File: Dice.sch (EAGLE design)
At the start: 14 parts, among them IC1 PIC12F629SN

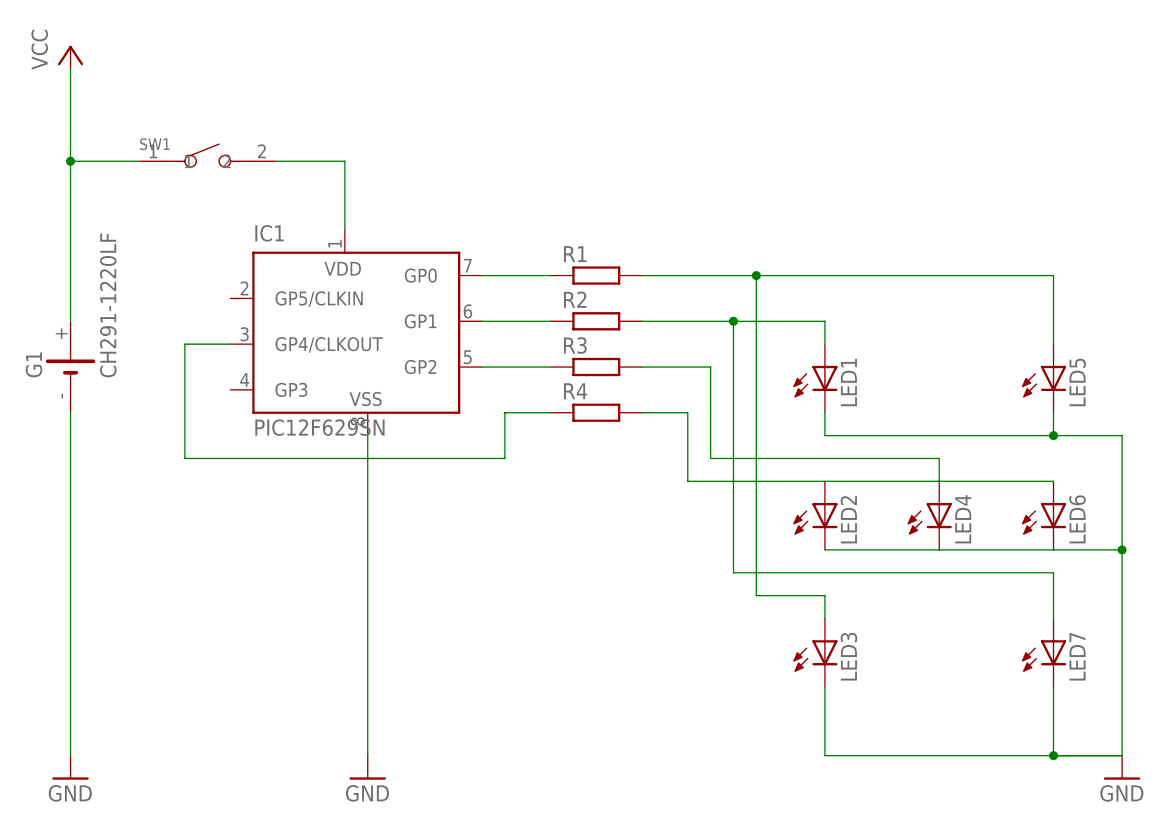
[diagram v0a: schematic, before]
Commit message: Always powered
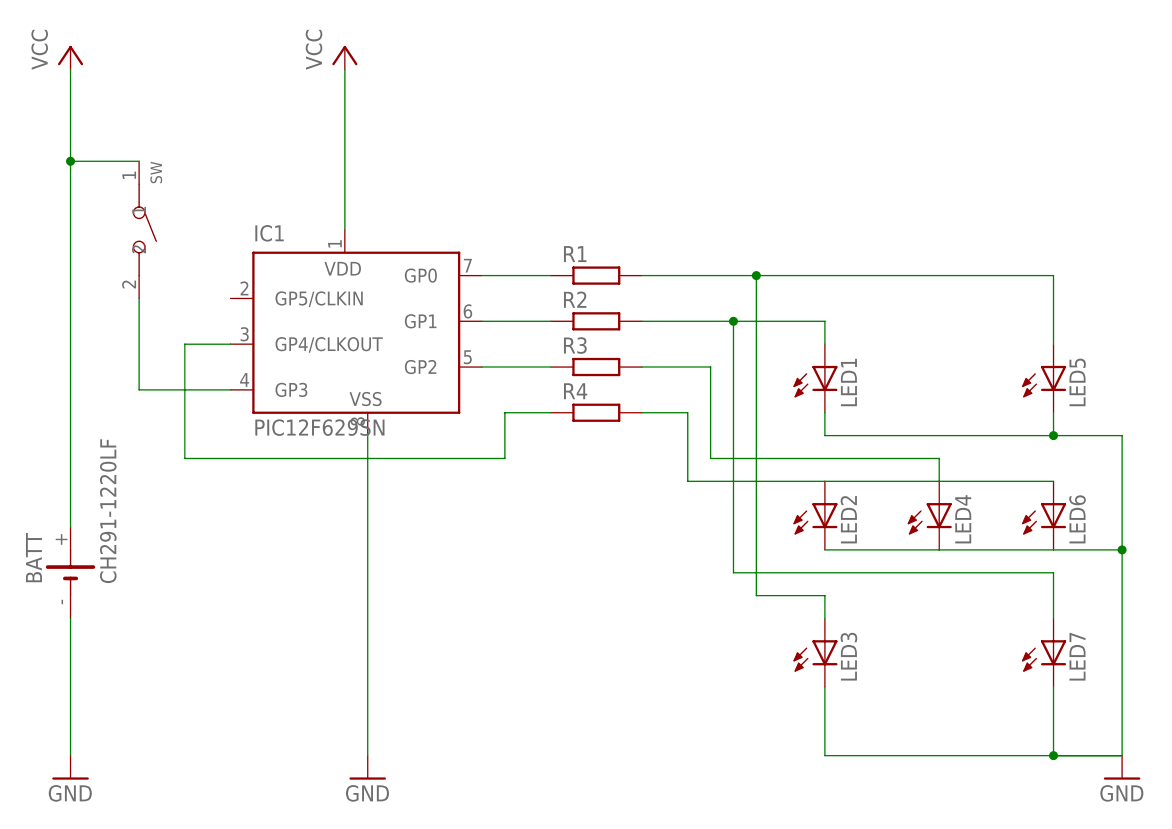
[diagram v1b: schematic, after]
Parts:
- removed G1: CH291-1220LF, battery:CH291-1220LF
- removed SW1: (no value), Seeed-OPL-Switch:SMD-BUTTON(2P-6.0X3.0X2.5MM)-DHT-1163S
- added BATT: CH291-1220LF, battery:CH291-1220LF
- added SW: (no value), Seeed-OPL-Switch:SMD-BUTTON(2P-6.0X3.0X2.5MM)-DHT-1163S
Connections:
- net N$11 renamed LED4
- net N$12 renamed LED2&6
- net N$2 renamed GP0
- net N$3 renamed GP1
- net N$4 renamed GP2
- net N$5 renamed GP4
- net N$6 renamed LED3&5
- net N$7 renamed LED1&7
- removed net N$1: IC1.VDD, SW1.2
- new net GP3: IC1.GP3, SW.2
- net GND: now also BATT.-; no longer G1.-
- net VCC: now also BATT.+, IC1.VDD, SW.1; no longer G1.+, SW1.1
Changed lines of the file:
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@@
 </classes>
 <parts>
-<part name="G1" library="battery" deviceset="CH291-1220LF" device=""/>
+<part name="BATT" library="battery" deviceset="CH291-1220LF" device=""/>
 <part name="GND1" library="supply1" deviceset="GND" device=""/>
 <part name="P+1" library="supply1" deviceset="VCC" device=""/>
@@
 <part name="R3" library="resistor" deviceset="R-EU_" device="R0805"/>
 <part name="R4" library="resistor" deviceset="R-EU_" device="R0805"/>
-<part name="SW1" library="Seeed-OPL-Switch" deviceset="SMD-BUTTON(2P-6.0X3.0X2.5MM)" device="-DHT-1163S"/>
+<part name="SW" library="Seeed-OPL-Switch" deviceset="SMD-BUTTON(2P-6.0X3.0X2.5MM)" device="-DHT-1163S"/>
 <part name="GND2" library="supply1" deviceset="GND" device=""/>
 <part name="GND3" library="supply1" deviceset="GND" device=""/>
+<part name="P+2" library="supply1" deviceset="VCC" device=""/>
 </parts>
 <sheets>
@@
 </plain>
 <instances>
-<instance part="G1" gate="G1" x="22.86" y="58.42" rot="R90"/>
+<instance part="BATT" gate="G1" x="22.86" y="35.56" rot="R90"/>
 <instance part="GND1" gate="1" x="22.86" y="12.7"/>
 <instance part="P+1" gate="VCC" x="22.86" y="93.98"/>
@@
 <instance part="R3" gate="G$1" x="81.28" y="58.42"/>
 <instance part="R4" gate="G$1" x="81.28" y="53.34"/>
-<instance part="SW1" gate="G$1" x="38.1" y="81.28"/>
+<instance part="SW" gate="G$1" x="30.48" y="73.66" rot="R270"/>
 <instance part="GND2" gate="1" x="55.88" y="12.7"/>
 <instance part="GND3" gate="1" x="139.7" y="12.7"/>
+<instance part="P+2" gate="VCC" x="53.34" y="93.98"/>
 </instances>
 <busses>
@@
 <segment>
 <pinref part="P+1" gate="VCC" pin="VCC"/>
-<pinref part="G1" gate="G1" pin="+"/>
+<pinref part="BATT" gate="G1" pin="+"/>
 <wire x1="22.86" y1="91.44" x2="22.86" y2="81.28" width="0.1524" layer="91"/>
-<pinref part="SW1" gate="G$1" pin="1"/>
-<wire x1="22.86" y1="81.28" x2="22.86" y2="63.5" width="0.1524" layer="91"/>
+<pinref part="SW" gate="G$1" pin="1"/>
+<wire x1="22.86" y1="81.28" x2="22.86" y2="40.64" width="0.1524" layer="91"/>
 <wire x1="22.86" y1="81.28" x2="30.48" y2="81.28" width="0.1524" layer="91"/>
 <junction x="22.86" y="81.28"/>
+</segment>
+<segment>
+<pinref part="P+2" gate="VCC" pin="VCC"/>
+<pinref part="IC1" gate="G$1" pin="VDD"/>
+<wire x1="53.34" y1="91.44" x2="53.34" y2="73.66" width="0.1524" layer="91"/>
 </segment>
 </net>
 <net name="GND" class="0">
 <segment>
-<pinref part="G1" gate="G1" pin="-"/>
+<pinref part="BATT" gate="G1" pin="-"/>
 <pinref part="GND1" gate="1" pin="GND"/>
-<wire x1="22.86" y1="53.34" x2="22.86" y2="15.24" width="0.1524" layer="91"/>
+<wire x1="22.86" y1="30.48" x2="22.86" y2="15.24" width="0.1524" layer="91"/>
 </segment>
 <segment>
@@
 </segment>
 </net>
-<net name="N$1" class="0">
+<net name="GP3" class="0">
 <segment>
-<pinref part="SW1" gate="G$1" pin="2"/>
-<pinref part="IC1" gate="G$1" pin="VDD"/>
-<wire x1="45.72" y1="81.28" x2="53.34" y2="81.28" width="0.1524" layer="91"/>
-<wire x1="53.34" y1="81.28" x2="53.34" y2="73.66" width="0.1524" layer="91"/>
+<pinref part="SW" gate="G$1" pin="2"/>
+<wire x1="30.48" y1="66.04" x2="30.48" y2="55.88" width="0.1524" layer="91"/>
+<pinref part="IC1" gate="G$1" pin="GP3"/>
+<wire x1="30.48" y1="55.88" x2="40.64" y2="55.88" width="0.1524" layer="91"/>
 </segment>
 </net>
-<net name="N$2" class="0">
+<net name="GP0" class="0">
 <segment>
 <pinref part="IC1" gate="G$1" pin="GP0"/>
@@
 </segment>
 </net>
-<net name="N$3" class="0">
+<net name="GP1" class="0">
 <segment>
 <pinref part="IC1" gate="G$1" pin="GP1"/>
@@
 </segment>
 </net>
-<net name="N$4" class="0">
+<net name="GP2" class="0">
 <segment>
 <pinref part="IC1" gate="G$1" pin="GP2"/>
@@
 </segment>
 </net>
-<net name="N$5" class="0">
+<net name="GP4" class="0">
 <segment>
 <pinref part="IC1" gate="G$1" pin="GP4/CLKOUT"/>
@@
 </segment>
 </net>
-<net name="N$6" class="0">
+<net name="LED3&amp;5" class="0">
 <segment>
 <pinref part="R1" gate="G$1" pin="2"/>
@@
 </segment>
 </net>
-<net name="N$7" class="0">
+<net name="LED1&amp;7" class="0">
 <segment>
 <pinref part="R2" gate="G$1" pin="2"/>
@@
 </segment>
 </net>
-<net name="N$11" class="0">
+<net name="LED4" class="0">
 <segment>
 <pinref part="R3" gate="G$1" pin="2"/>
@@
 </segment>
 </net>
-<net name="N$12" class="0">
+<net name="LED2&amp;6" class="0">
 <segment>
 <pinref part="R4" gate="G$1" pin="2"/>
